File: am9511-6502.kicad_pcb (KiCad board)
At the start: 2 copper layers, 82.1 x 67.5 mm, 24 parts, among them J1 Conn_01x18_Pin, U1 AM9511A, U2 ATF16V8B, U3 74HC112, U4 ADA-TPS61040, U5 74HC123, X1 4 MHz

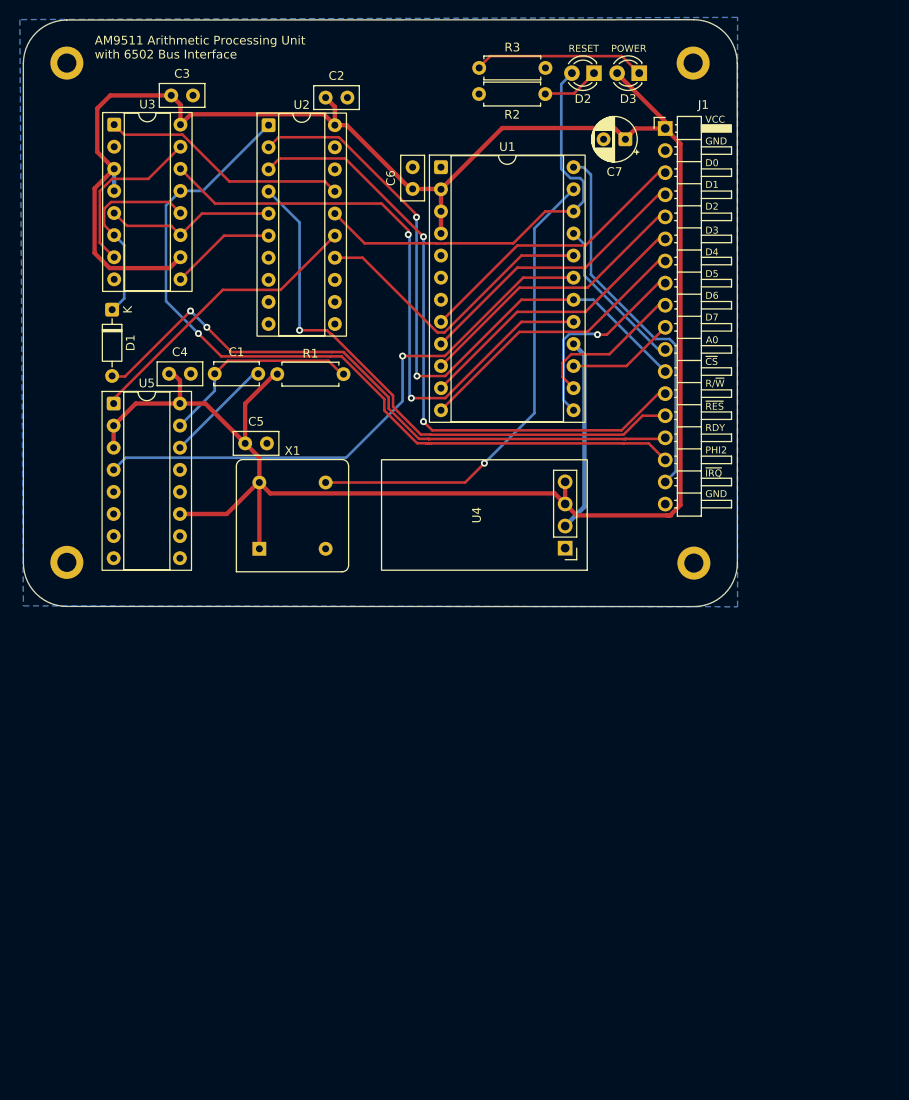
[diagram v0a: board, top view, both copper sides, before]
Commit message: Initial PAL-2 version
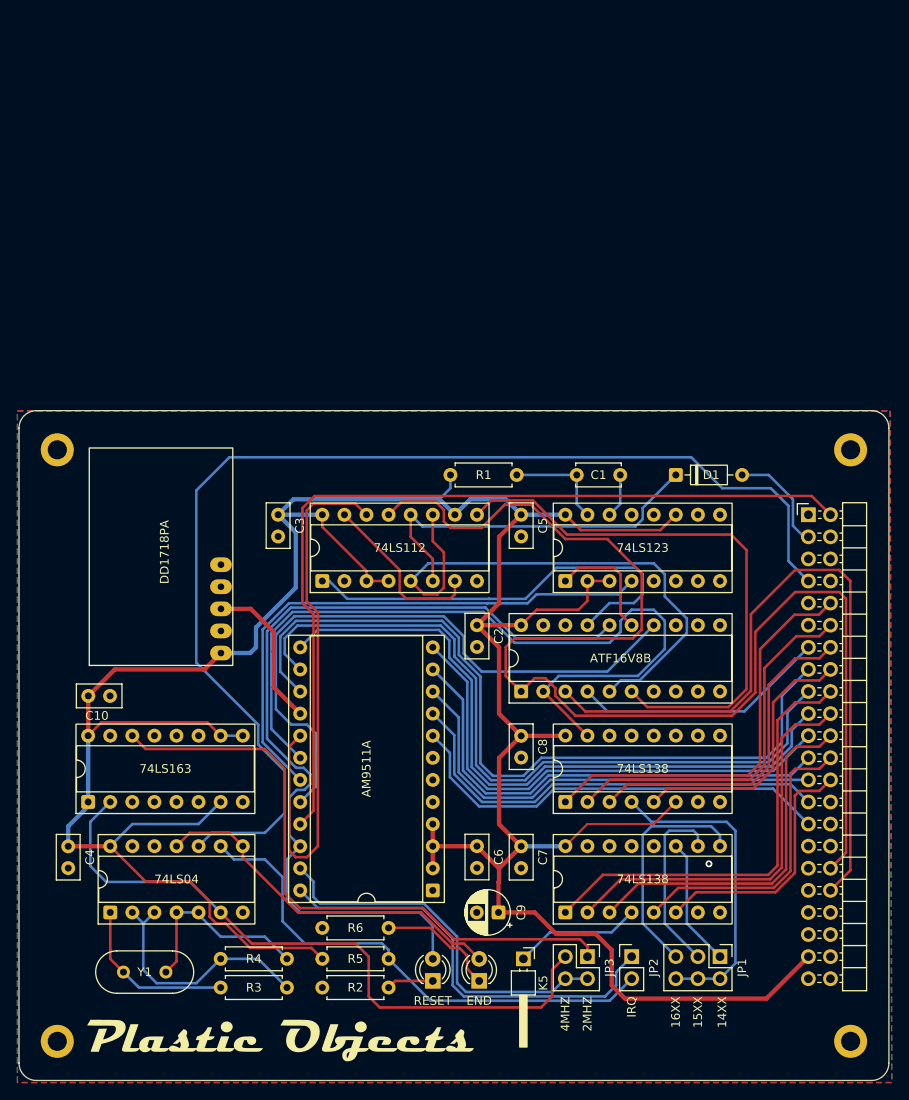
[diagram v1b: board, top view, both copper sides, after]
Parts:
- removed X1: 4 MHz, Oscillator:Oscillator_DIP-8
- added C10: 100nF, Capacitor_THT:C_Disc_D5.0mm_W2.5mm_P2.50mm, F.Cu at (107.5, 97.8)
- added C8: 100nF, Capacitor_THT:C_Disc_D5.0mm_W2.5mm_P2.50mm, F.Cu at (157.2, 102.4)
- added C9: 1µF, Capacitor_THT:CP_Radial_D5.0mm_P2.50mm, F.Cu at (154.6, 122.7)
- added G***: LOGO, LOGO, F.Cu at (129.5, 137.4)
- added J2: K5, Connector_PinHeader_2.54mm:PinHeader_1x01_P2.54mm_Horizontal, F.Cu at (157.5, 128.0)
- added JP1: BASE_ADDR, Connector_PinHeader_2.54mm:PinHeader_2x03_P2.54mm_Vertical, F.Cu at (180.1, 127.8)
- added JP2: IRQ_ENABLE, Connector_PinHeader_2.54mm:PinHeader_1x02_P2.54mm_Vertical, F.Cu at (169.9, 127.8)
- added JP3: CLOCK, Connector_PinHeader_2.54mm:PinHeader_2x02_P2.54mm_Vertical, F.Cu at (164.8, 127.8)
- added R4: 2K2, Resistor_THT:R_Axial_DIN0207_L6.3mm_D2.5mm_P7.62mm_Horizontal, F.Cu at (130.3, 128.0)
- added R5: 2K7, Resistor_THT:R_Axial_DIN0207_L6.3mm_D2.5mm_P7.62mm_Horizontal, F.Cu at (134.4, 128.0)
- added R6: 470, Resistor_THT:R_Axial_DIN0207_L6.3mm_D2.5mm_P7.62mm_Horizontal, F.Cu at (134.4, 124.5)
- added U6: 74LS138, Package_DIP:DIP-16_W7.62mm_Socket, F.Cu at (162.3, 122.7)
- added U7: 74LS138, Package_DIP:DIP-16_W7.62mm_Socket, F.Cu at (162.3, 110.0)
- added U8: 74LS04, Package_DIP:DIP-14_W7.62mm_Socket, F.Cu at (110.0, 122.7)
- added U9: 74LS163, Package_DIP:DIP-16_W7.62mm_Socket, F.Cu at (107.4, 110.0)
- added Y1: 4Mhz, Crystal:Crystal_HC49-4H_Vertical, F.Cu at (111.5, 129.5)
- C7: value 1µF -> 100nF; footprint Capacitor_THT:CP_Radial_D5.0mm_P2.50mm -> Capacitor_THT:C_Disc_D5.0mm_W2.5mm_P2.50mm
- D2: value YELLOW -> RESET
- D3: value BLUE -> END
- J1: value Conn_01x18_Pin -> PAL2_Expansion; footprint am9511-6502-footprints:PinHeader_1x18_P2.54mm_Horizontal -> Connector_PinHeader_2.54mm:PinHeader_2x22_P2.54mm_Horizontal
- R3: value 1K -> 2K2
- U3: value 74HC112 -> 74LS112
- U4: value ADA-TPS61040 -> DD1718PA; footprint am9511-6502-footprints:ADA-TPS61040 -> am9511-6502-footprints:DD1718PA
- U5: value 74HC123 -> 74LS123
- moved H1 112.5 mm to (103.9, 137.5)
- moved R3 108.0 mm to (130.3, 131.3), turned to 180 degrees
- moved D2 106.0 mm to (147.1, 130.6), turned to 90 degrees
- moved D3 106.0 mm to (152.4, 130.6), turned to 90 degrees
- moved R2 105.9 mm to (134.4, 131.3), turned to 0 degrees
- moved H3 91.0 mm to (195.1, 69.5)
- moved H2 85.6 mm to (103.9, 69.5)
- moved U1 83.1 mm to (147.1, 120.1), turned to 180 degrees
- moved C7 82.2 mm to (157.2, 115.1), turned to -90 degrees
- moved C6 75.9 mm to (152.1, 115.1), turned to -90 degrees
- moved U2 71.3 mm to (157.2, 97.3), turned to 90 degrees
- moved D1 67.5 mm to (175.0, 72.4), turned to 0 degrees
- moved C2 63.1 mm to (152.1, 89.7), turned to -90 degrees
- moved H4 57.9 mm to (195.1, 137.5)
- moved U3 57.7 mm to (134.4, 84.6), turned to 90 degrees
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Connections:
- D3 pad 2: VCC -> Net-(D3-A)
- J1 pad 1: VCC -> /PAL-2 Interface/SYNC
- J1 pad 10: /D7 -> /PAL-2 Interface/AB4
- J1 pad 11: /A0 -> /PAL-2 Interface/NMI
- J1 pad 12: /~{CS} -> /PAL-2 Interface/AB5
- J1 pad 13: /R/~{W} -> /~{RST}
- J1 pad 14: /~{RESET} -> /PAL-2 Interface/AB6
- J1 pad 15: /RDY -> /D7
- J1 pad 16: /PHI2 -> /PAL-2 Interface/AB7
- J1 pad 17: /~{IRQ} -> /D6
- J1 pad 18: GND -> /PAL-2 Interface/AB8
- J1 pad 2: GND -> /A0
- J1 pad 3: /D0 -> /RDY
- J1 pad 4: /D1 -> /PAL-2 Interface/AB1
- J1 pad 5: /D2 -> /PAL-2 Interface/PHI1
- J1 pad 6: /D3 -> /PAL-2 Interface/AB2
- J1 pad 7: /D4 -> /~{IRQ}
- J1 pad 8: /D5 -> /PAL-2 Interface/AB3
- J1 pad 9: /D6 -> /PAL-2 Interface/SO
- R2 pad 1: Net-(D2-K) -> GND
- R2 pad 2: GND -> Net-(D2-K)
- R3 pad 1: Net-(D3-K) -> Net-(R3-Pad1)
- R3 pad 2: GND -> Net-(R3-Pad2)
- U1 pad 23: Net-(U1-CLK) -> /CLOCK
- U1 pad 24: /~{IRQ} -> Net-(JP2-A)
- U2 pad 4: /~{RESET} -> /~{RST}
- U4 pad 1: GND -> VCC
- U4 pad 2: Net-(U1-VDD) -> GND
- U4 pad 3: VCC -> Net-(U1-VDD)
- U4 pad 4: VCC -> GND
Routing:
- net /~{IRQ}: track 43.2 -> 134.3 mm
- net /A0: track 17.4 -> 99.7 mm
- net /D7: track 12.4 -> 91.3 mm
- net Net-(JP3-Pin_3): track 0.00 -> 76.5 mm
- net Net-(JP3-Pin_1): track 0.00 -> 71.9 mm
- net VCC: track 281.8 -> 352.6 mm
- net /D6: track 18.0 -> 85.8 mm
- net /~{RESET}: track 66.1 -> 0.00 mm, vias 1 -> 0
- net /RDY: track 73.6 -> 12.4 mm, vias 2 -> 0
- net Net-(JP2-B): track 0.00 -> 59.2 mm
- net /D5: track 23.0 -> 78.1 mm, vias 1 -> 0
- net Net-(U1-CLK): track 54.9 -> 0.00 mm, vias 1 -> 0
- net /PHI2: track 92.3 -> 147.2 mm, vias 1 -> 0
- net /Q2: track 12.2 -> 64.8 mm
- net /RESET: track 49.0 -> 100.5 mm
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- added copper zone on F.Cu, net GND
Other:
- board size 82.1 x 67.5 mm -> 100 x 77 mm
- board text added: "14XX"
- board text added: "15XX"
- board text added: "16XX"
- board text added: "2MHZ"
- board text added: "4MHZ"
- board text added: "IRQ"
- board text removed: "A0"
- board text removed: "AM9511 Arithmetic Processing Unit with 6502 Bus Interface"
- board text removed: "D0"
- board text removed: "D1"
- board text removed: "D2"
- board text removed: "D3"
- board text removed: "D4"
- board text removed: "D5"
- board text removed: "D6"
- board text removed: "D7"
- board text removed: "Designed in Blacksburg, Virginia, USA"
- board text removed: "GND"
- board text removed: "PHI2"
- board text removed: "POWER"
- board text removed: "R/~{W}"
- board text removed: "RDY"
- board text removed: "RESET"
- board text removed: "VCC"
- board text removed: "~{CS}"
- board text removed: "~{IRQ}"
- board text removed: "~{RES}"
